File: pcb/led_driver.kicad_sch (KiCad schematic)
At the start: 10 parts, among them Q1 PMOS, U1 LTC3454EDD_TRPBF, U2 MCP73831-2-OT

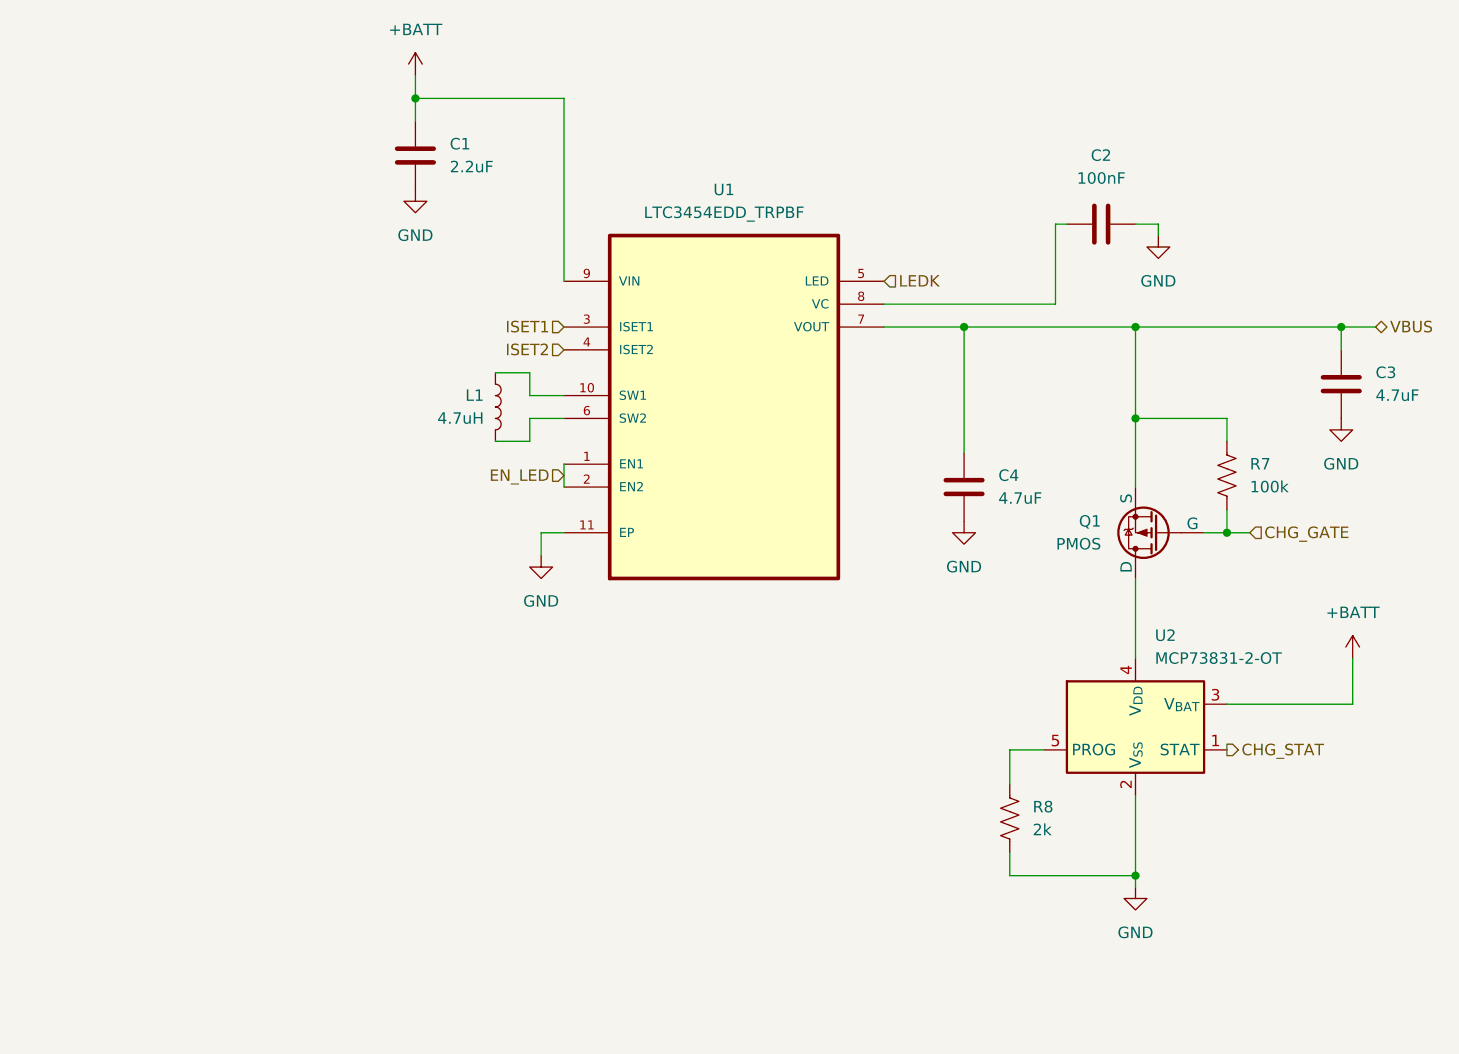
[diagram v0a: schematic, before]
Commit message: rev0 done
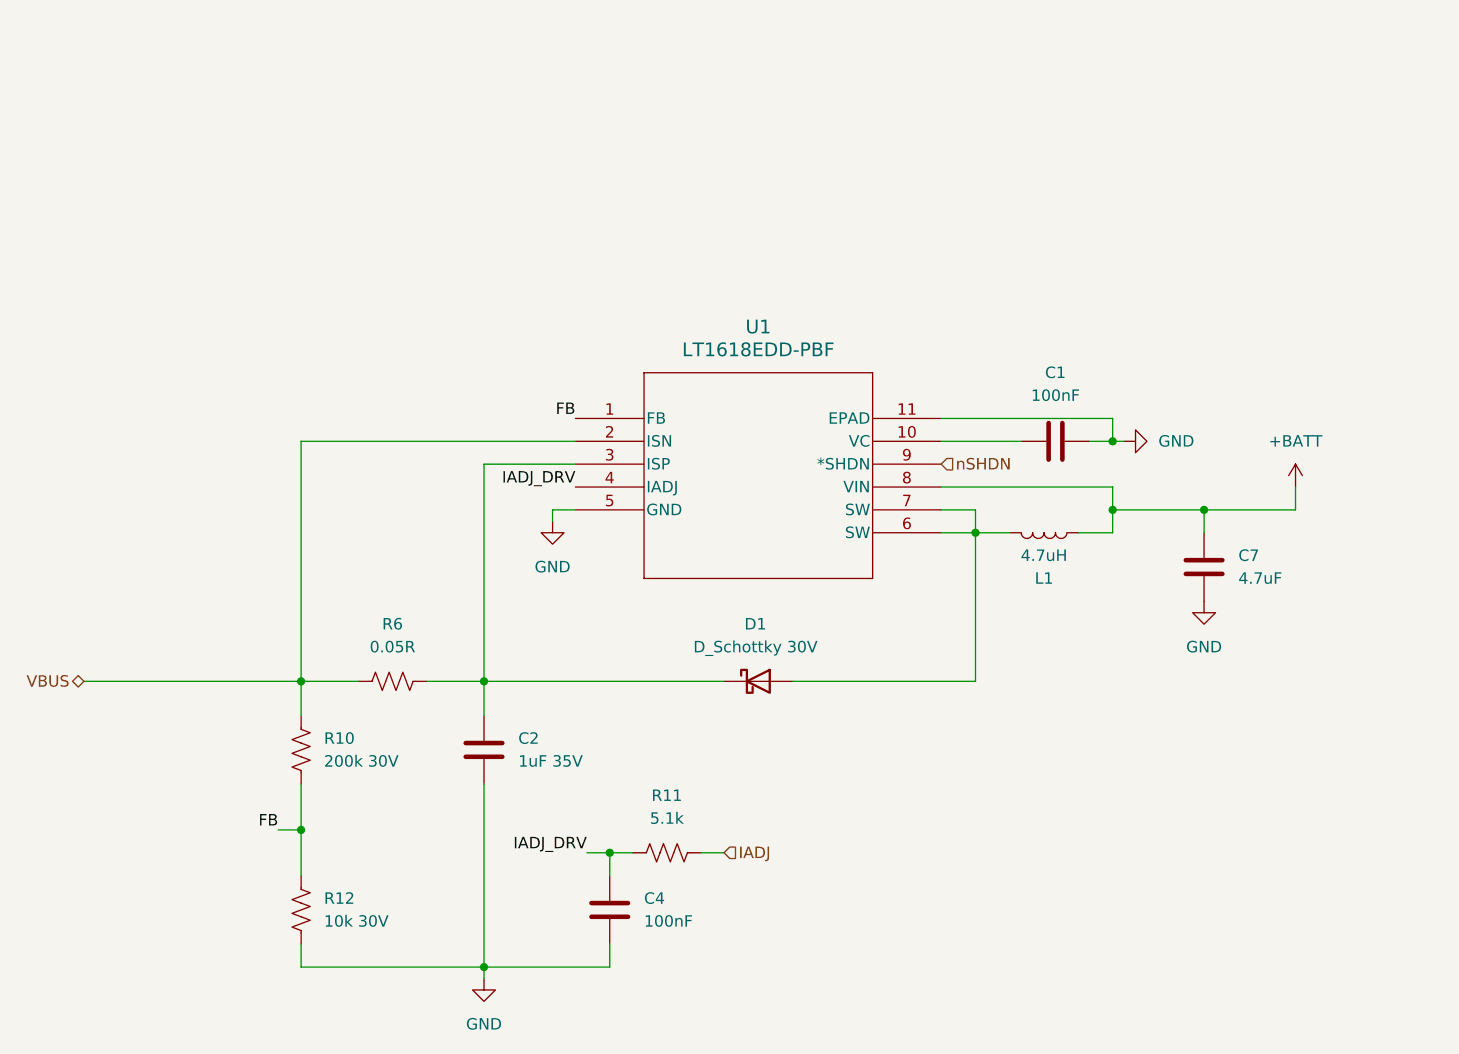
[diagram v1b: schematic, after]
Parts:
- removed C3: 4.7uF, Capacitor_SMD:C_0402_1005Metric, symbol Device:C
- removed Q1: PMOS, Package_TO_SOT_SMD:SOT-23-3, symbol Simulation_SPICE:PMOS
- removed R7: 100k, Resistor_SMD:R_0402_1005Metric, symbol Device:R_US
- removed R8: 2k, Resistor_SMD:R_0402_1005Metric, symbol Device:R_US
- removed U1: LTC3454EDD_TRPBF, footprints:DFN300X300X80-11N, symbol LTC3454EDD_TRPBF:LTC3454EDD_TRPBF
- removed U2: MCP73831-2-OT, Package_TO_SOT_SMD:SOT-23-5, symbol Battery_Management:MCP73831-2-OT
- added C7: 4.7uF, Capacitor_SMD:C_0402_1005Metric, symbol Device:C
- added D1: D_Schottky 30V, Diode_SMD:D_SOD-123, symbol Device:D_Schottky
- added R10: 200k 30V, Resistor_SMD:R_0402_1005Metric, symbol Device:R_US
- added R11: 5.1k, Resistor_SMD:R_0402_1005Metric, symbol Device:R_US
- added R12: 10k 30V, Resistor_SMD:R_0402_1005Metric, symbol Device:R_US
- added R6: 0.05R, Resistor_SMD:R_1206_3216Metric, symbol Device:R_US
- added U1: LT1618EDD-PBF, DFN-10_DD_LIT, symbol LT1618:LT1618EDD-PBF
- C1: value 2.2uF -> 100nF
- C2: value 100nF -> 1uF 35V; footprint Capacitor_SMD:C_0402_1005Metric -> Capacitor_SMD:C_0603_1608Metric
- C4: value 4.7uF -> 100nF
- L1: footprint Inductor_SMD:L_Changjiang_FNR4020S -> Inductor_SMD:L_Changjiang_FNR4030S
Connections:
- net +BATT: now also L1.2, C7.1, U1.8 (VIN); no longer C1.1
- net GND: now also C2.2, C7.2, R12.1, U1.11 (EPAD), U1.5 (GND); no longer C2.1
- net VBUS: now also R10.2, R6.2, U1.2 (ISN); no longer C4.1
- net at L1.1: now also D1.2 (A), U1.6 (SW), U1.7 (SW)
- new net: C2.1, D1.1 (K), R6.1, U1.3 (ISP)
- new net: C1.1, U1.10 (VC)
- new net FB: R10.1, R12.2, U1.1 (FB)
- new net IADJ: R11.1
- new net IADJ_DRV: C4.1, R11.2, U1.4 (IADJ)
- new net nSHDN: U1.9 (*SHDN)
